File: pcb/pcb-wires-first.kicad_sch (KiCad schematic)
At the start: 50 parts, among them J10 Conn_01x02, J11 Conn_01x02, J2 Conn_01x02, J5 Conn_01x04, J6 Conn_01x04, J7 Conn_01x04, J9 Conn_01x02, SW1 off-2, SW2 on-2, SW3 on-1, SW4 off-1, SW5 on-3, SW6 off-3, U1 SLG47115V, U2 SLG46826V, U3 R-78C3.3-1.0

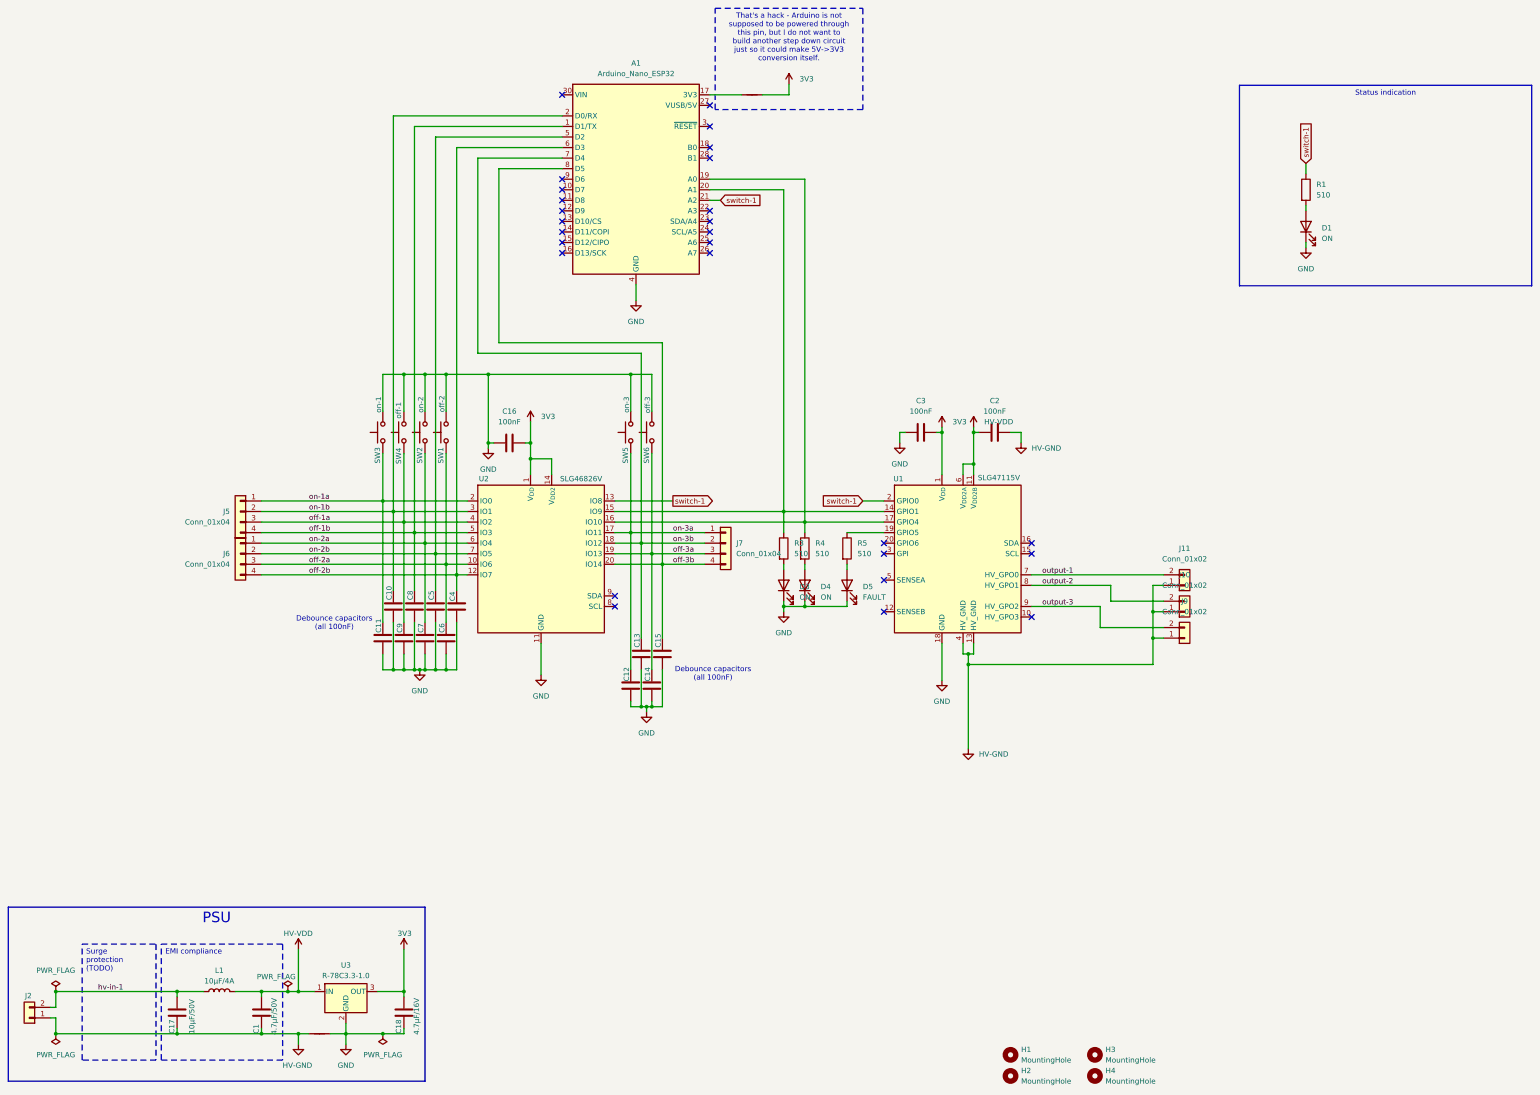
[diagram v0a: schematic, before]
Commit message: Tidying up schematic.
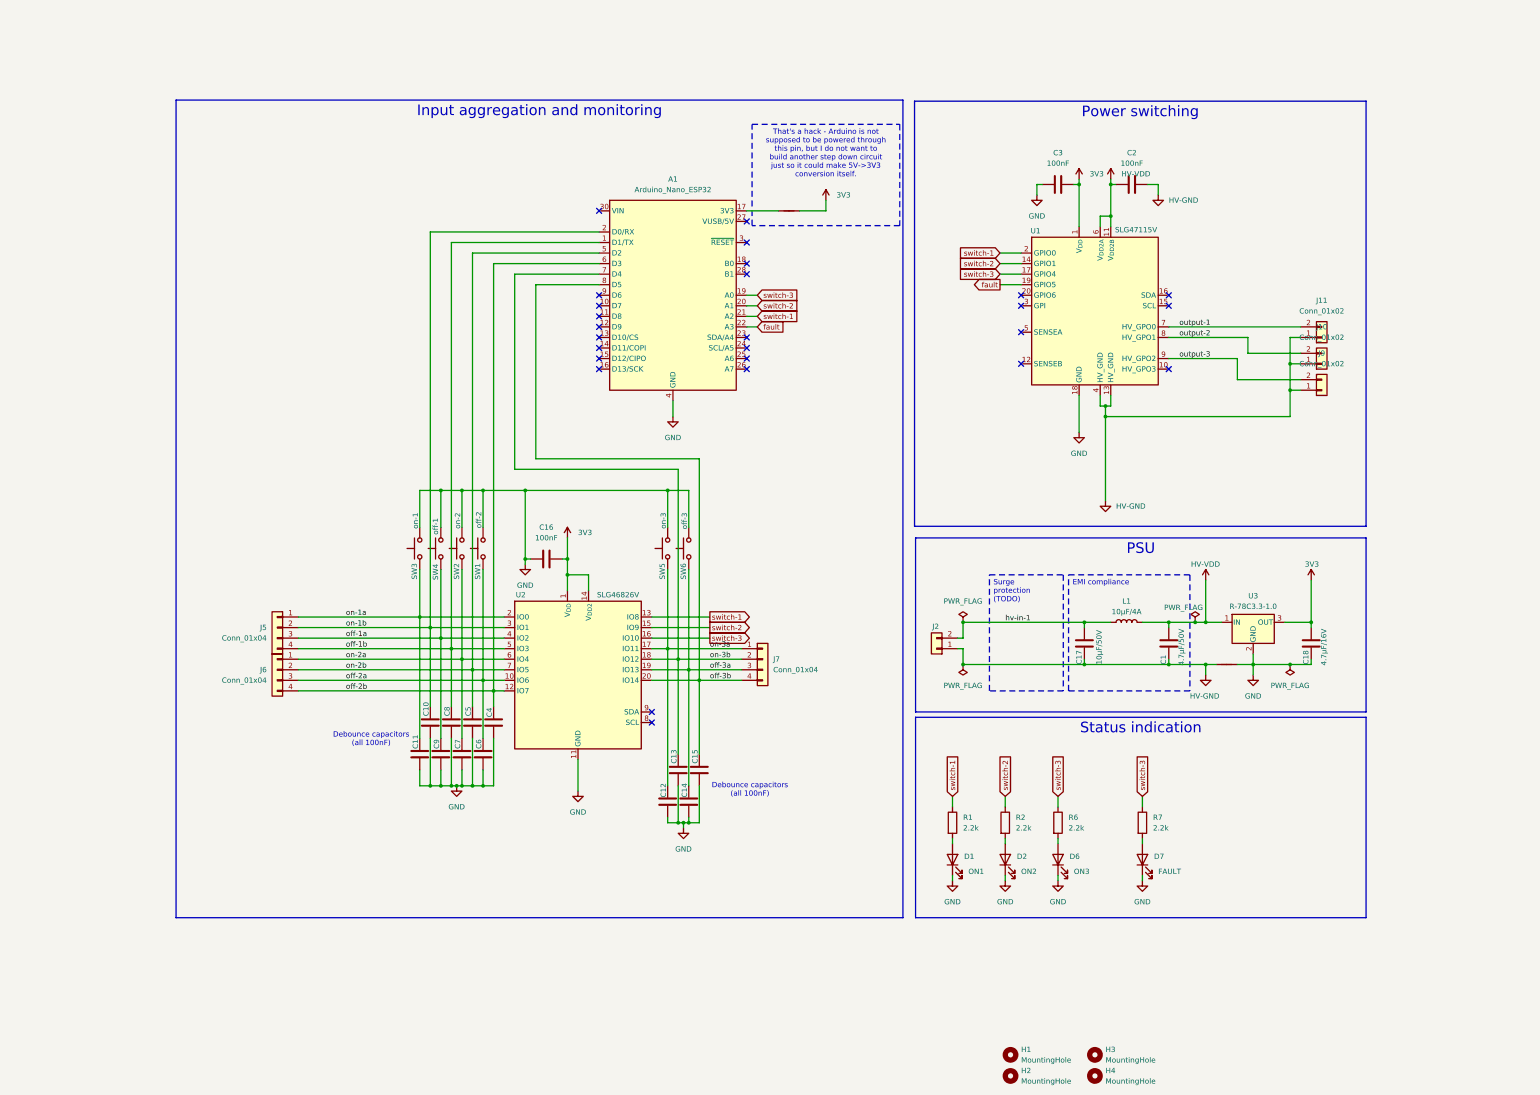
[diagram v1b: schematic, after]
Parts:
- removed D3, D4: ON, Diode_SMD:D_0603_1608Metric, symbol Device:LED
- removed D5: FAULT, Diode_SMD:D_0603_1608Metric, symbol Device:LED
- removed R3, R4, R5: 510, Resistor_SMD:R_0603_1608Metric, symbol Device:R
- added D2: ON2, Diode_SMD:D_0603_1608Metric, symbol Device:LED
- added D6: ON3, Diode_SMD:D_0603_1608Metric, symbol Device:LED
- added D7: FAULT, Diode_SMD:D_0603_1608Metric, symbol Device:LED
- added R2, R6, R7: 2.2k, Resistor_SMD:R_0603_1608Metric, symbol Device:R
- D1: value ON -> ON1
- R1: value 510 -> 2.2k
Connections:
- net GND: now also D2.1 (K), D6.1 (K), D7.1 (K)
- net fault: now reaches U1.19 (GPIO5)
- net fault: now also A1.22 (A3)
- net switch-3: now reaches A1.19 (A0), U1.17 (GPIO4), U2.16 (IO10)
- net switch-3: now also R6.1, R7.1
- net switch-2: now reaches A1.20 (A1), U1.14 (GPIO1), U2.15 (IO9)
- net switch-2: now also R2.1
- new net: D7.2 (A), R7.2
- new net: D6.2 (A), R6.2
- new net: D2.2 (A), R2.2
- no-connect marks 27 -> 26
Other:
- moved on the sheet: A1, C1, C10, C11, C12, C13, C14, C15, C16, C17, C18, C2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
